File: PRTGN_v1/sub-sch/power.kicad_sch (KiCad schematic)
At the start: 20 parts, among them IC1 TPS565242DRLR, J2 Barrel_Jack, J3 Screw_Terminal_01x02, J4 Screw_Terminal_01x02, Q1 Q_PMOS, Q2 Q_PMOS, SW1 SW_DPDT_x2

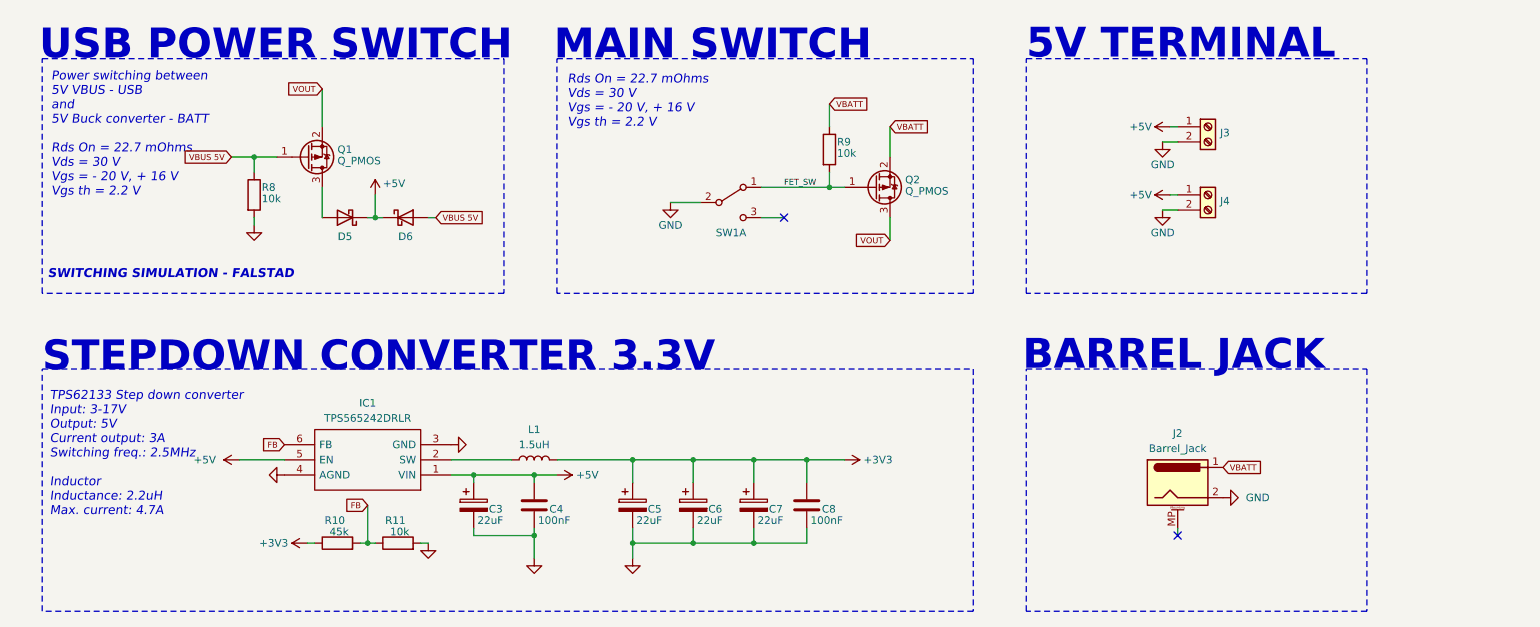
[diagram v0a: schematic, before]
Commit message: PCV updates
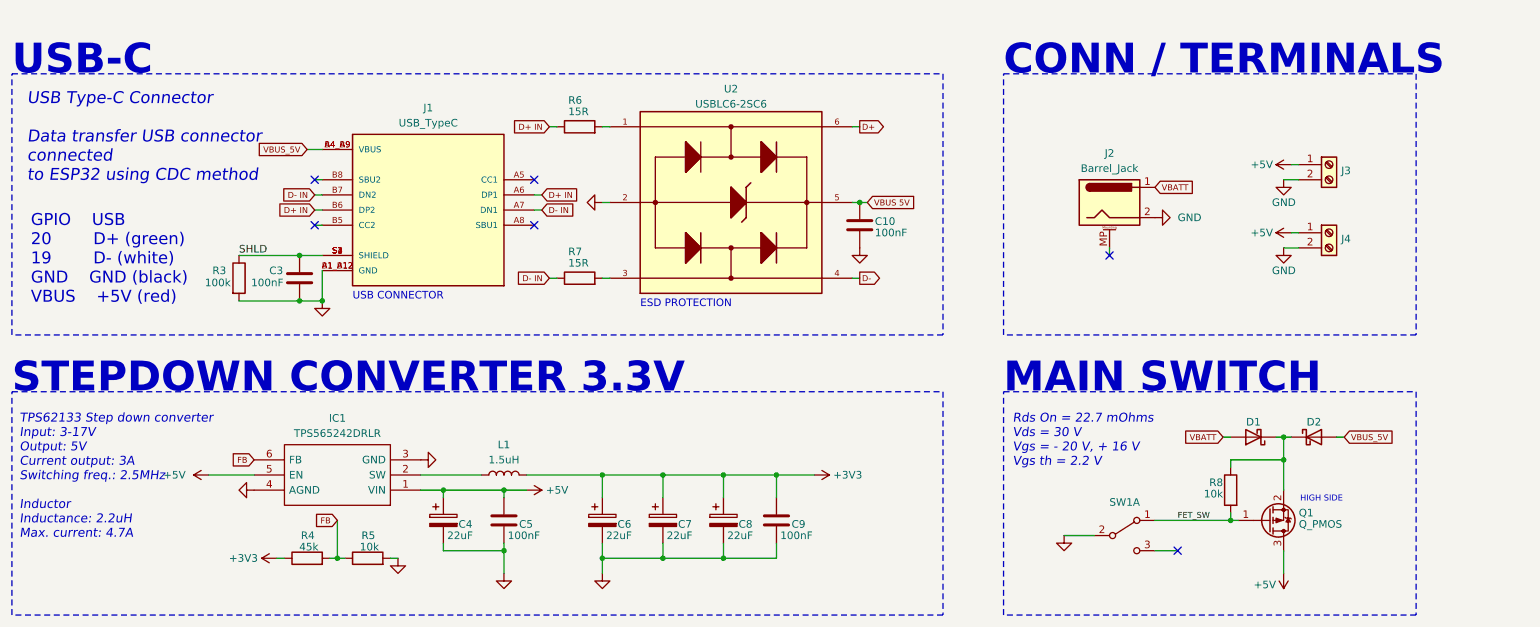
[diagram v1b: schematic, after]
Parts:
- removed Q1: Q_PMOS, Package_TO_SOT_SMD:SOT-23-3, symbol Device:Q_PMOS_GSD
- removed R8: 10k, Resistor_SMD:R_0805_2012Metric_Pad1.20x1.40mm_HandSolder, symbol Device:R
- added C10, C3: 100nF, Capacitor_SMD:C_0805_2012Metric_Pad1.18x1.45mm_HandSolder, symbol Device:C
- added J1: USB_TypeC, sumec_brd:HRO_TYPE-C-31-M-12, symbol sumec_sch_lib:USB_TypeC
- added R3: 100k, Resistor_SMD:R_0805_2012Metric_Pad1.20x1.40mm_HandSolder, symbol Device:R
- added R6, R7: 15R, Resistor_SMD:R_0805_2012Metric_Pad1.20x1.40mm_HandSolder, symbol Device:R
- added U2: USBLC6-2SC6, Package_TO_SOT_SMD:TSOT-23-6_HandSoldering, symbol sumec_library:USBLC6-2SC6
- renumbered C3 to C4, C4 to C5, C5 to C6, C6 to C7, C7 to C8, C8 to C9, D5 to D1, D6 to D2, Q2 to Q1, R10 to R4, R11 to R5, R9 to R8
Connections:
- net VOUT is gone; now on net +5V: Q1.3 (D)
- net +5V: no longer D1.1 (K), D2.1 (K)
- net GND: now also C10.2, C3.1, J1.A1_B12 (GND), J1.B1_A12 (GND), R3.2, U2.2
- net VBATT: now also D1.2 (A); no longer Q1.2 (S), R8.1
- net VBUS 5V: now also C10.1, U2.5; no longer D2.2 (A)
- new net: D1.1 (K), D2.1 (K), Q1.2 (S), R8.1
- new net: R6.2, U2.1
- new net: R7.2, U2.3
- new net D+: U2.6
- new net D+ IN: J1.A6 (DP1), J1.B6 (DP2), R6.1
- new net D-: U2.4
- new net D- IN: J1.A7 (DN1), J1.B7 (DN2), R7.1
- new net SHLD: C3.2, J1.S1 (SHIELD), J1.S2 (SHIELD), J1.S3 (SHIELD), J1.S4 (SHIELD), R3.1
- new net VBUS_5V: D2.2 (A), J1.A4_B9 (VBUS), J1.B4_A9 (VBUS)
- no-connect marks 2 -> 6
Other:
- note added: "CONN / TERMINALS"
- note added: "ESD PROTECTION"
- note added: "GPIO USB 20 D+ (green) 19 D- (white) GND GND (black) VBUS +5V (red)"
- note added: "HIGH SIDE"
- note added: "USB CONNECTOR"
- note added: "USB Type-C Connector Data transfer USB connector connected to ESP32 using CDC method"
- note added: "USB-C"
- note removed: "5V TERMINAL"
- note removed: "BARREL JACK"
- note removed: "Power switching between 5V VBUS - USB and 5V Buck converter - BATT"
- note removed: "SWITCHING SIMULATION - FALSTAD"
- note removed: "USB POWER SWITCH"
- moved on the sheet: C4, C5, C6, C7, C8, C9, D1, D2, IC1, J2, J3, J4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
